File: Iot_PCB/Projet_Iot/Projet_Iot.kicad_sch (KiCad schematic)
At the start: 19 parts, among them J10 110990030, J15 110990030, J16 110990030, J17 110990030, J18 110990030, J23 110990030, J24 110990030, J6 110990030, J7 110990030, J8 110990030, J9 110990030, U11 FDC6326L, U6 uPesy_ESP32_Wroom_Low_Power_D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

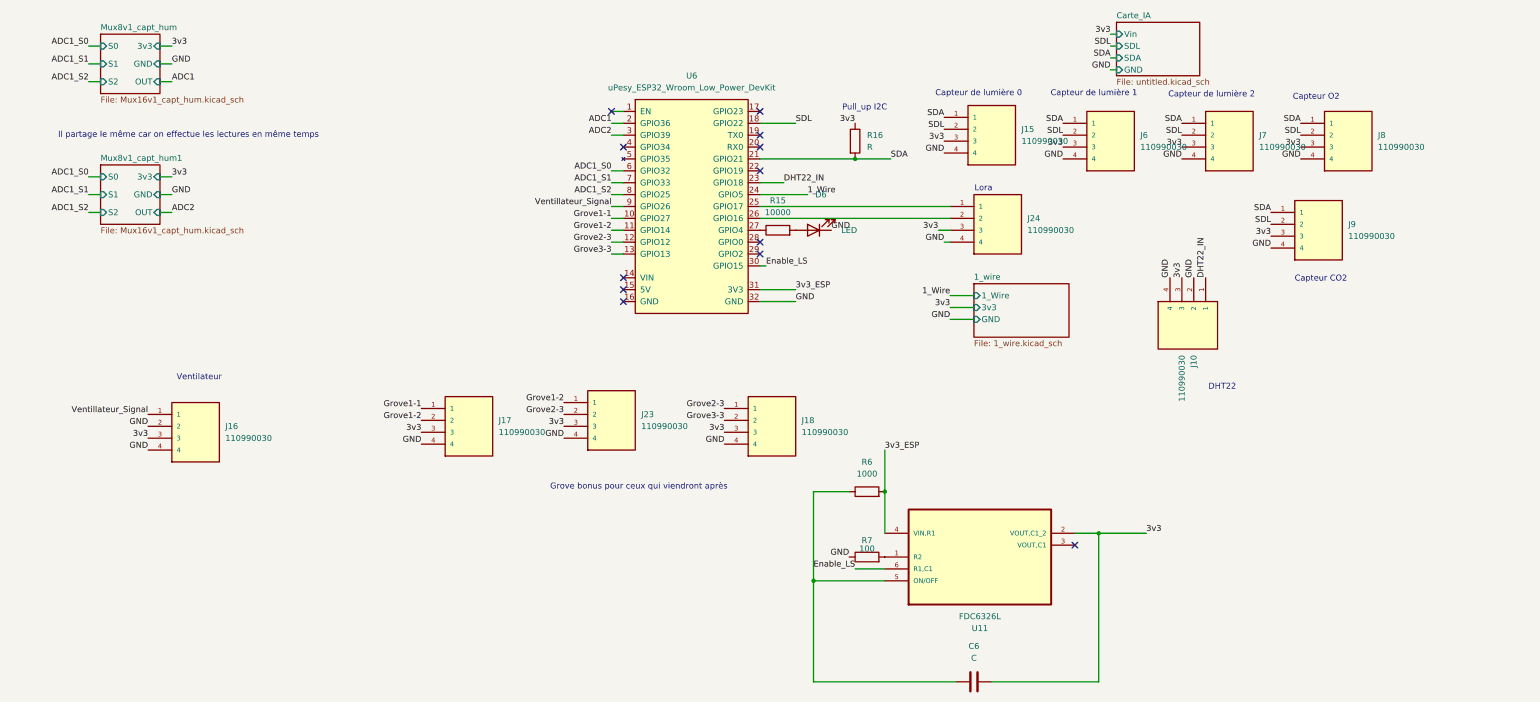
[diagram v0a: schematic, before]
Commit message: pcb and schematic up to date
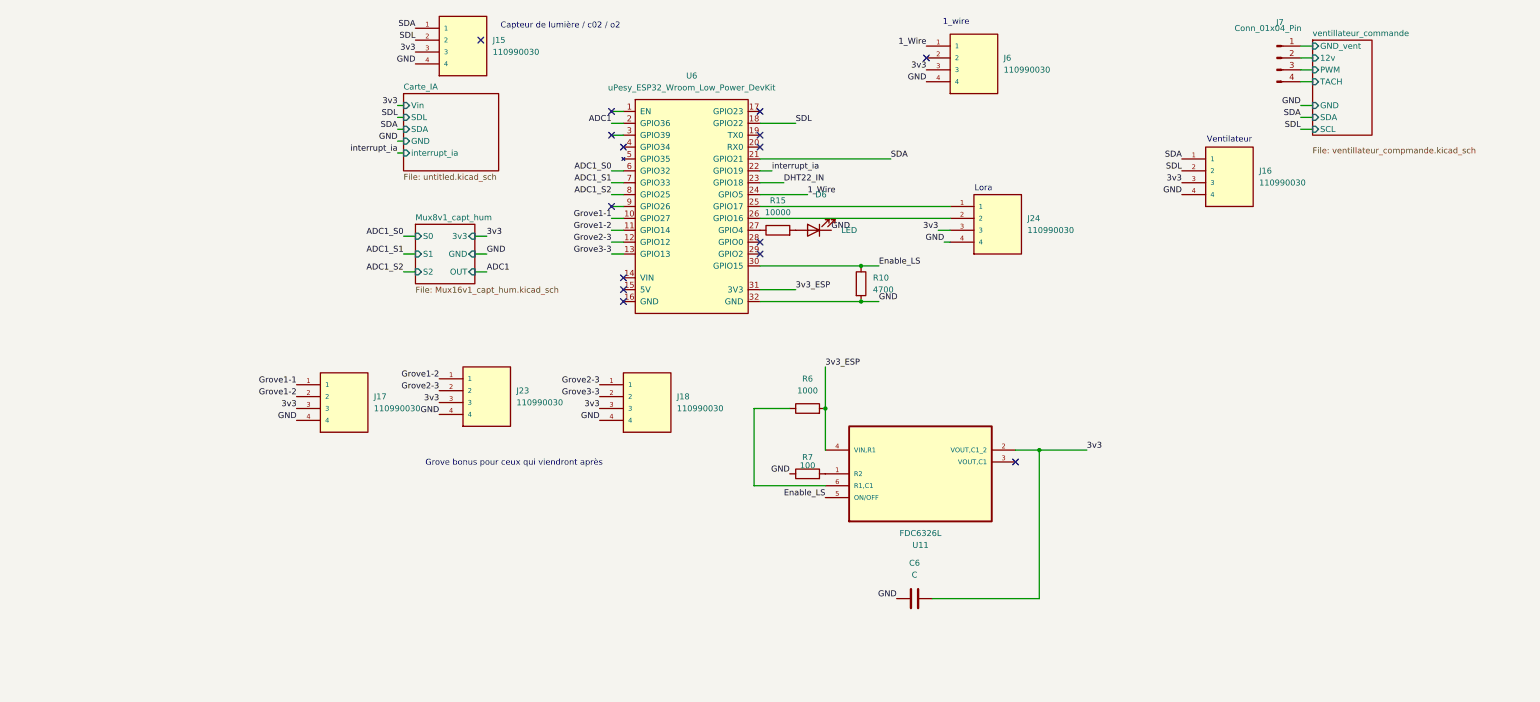
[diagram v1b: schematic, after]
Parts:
- removed J10, J7, J8, J9: 110990030, Grove:SEEED_110990030, symbol grove:110990030
- removed R16: R, Resistor_THT:R_Axial_DIN0207_L6.3mm_D2.5mm_P10.16mm_Horizontal, symbol Device:R
- added J7: Conn_01x04_Pin, symbol Connector:Conn_01x04_Pin
- added R10: 4700, symbol Device:R
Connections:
- net 1_Wire: now also J6.1
- net Enable_LS: now also U11.5 (ON/OFF), R10.1; no longer U11.6 (R1,C1)
- net GND: now also C6.1, R10.2; no longer J16.2
- net SDA: now also J16.1; no longer J6.1
- net SDL: now also J16.2; no longer J6.2
- net interrupt_ia: now reaches U6.22 (GPIO19)
- net ADC2: no longer names the net of U6.3 (GPIO39)
- net Ventillateur_Signal: no longer names the net of U6.9 (GPIO26)
- net Ventillateur_Signal: no longer J16.1
- new net: R6.1, U11.6 (R1,C1)
- new net ventillateur_commande/12v: J7.2 (Pin_2)
- new net ventillateur_commande/GND_vent: J7.1 (Pin_1)
- new net ventillateur_commande/PWM: J7.3 (Pin_3)
- new net ventillateur_commande/TACH: J7.4 (Pin_4)
- no-connect marks 12 -> 15
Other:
- removed sheet 1_wire
- removed sheet Mux8v1_capt_hum1
- added sheet ventillateur_commande (ventillateur_compmande.kicad_sch)
- sheet Carte_IA ports: added interrupt_ia; removed none
- note added: "1_wire"
- note added: "Capteur de lumière / c02 / o2"
- note removed: "Capteur CO2"
- note removed: "Capteur O2"
- note removed: "Capteur de lumière 0"
- note removed: "Capteur de lumière 1"
- note removed: "Capteur de lumière 2"
- note removed: "DHT22"
- note removed: "Il partage le même car on effectue les lectures en même temps"
- note removed: "Pull_up I2C"
- moved on the sheet: C6, J15, J16, J17, J18, J23, R6, R7, U11
